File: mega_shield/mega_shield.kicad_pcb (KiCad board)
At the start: 2 copper layers, 296 parts, among them J11 T4040014031-000, J13 T4040014031-000, J14 1757242, J15 1757242, J17 T4040014031-000, J19 T4040014031-000, J20 T4140012121-000, J3 1757271, J9 T4040014031-000, Q1 2SK3018, Q10 2SK3018, Q11 2SK3018, Q12 2SK3018, Q13 2SK3018, Q14 2SK3018, Q15 2SK3018, Q16 2SK3018, Q17 2SK3018, Q18 2SK3018, Q19 2SK3018, Q2 2SK3018, Q20 2SK3018, Q21 2SK3018, Q22 2SK3018, Q23 2SK3018, Q24 2SK3018, Q25 2SK3018, Q26 2SK3018, Q27 2SK3018, Q28 2SK3018, Q29 2SK3018, Q3 2SK3018, Q30 2SK3018, Q31 2SK3018, Q32 2SK3018, Q33 2SK3018, Q34 2SK3018, Q35 2SK3018, Q36 2SK3018, Q37 2SK3018, Q38 2SK3018, Q39 2SK3018, Q4 2SK3018, Q40 2SK3018, Q41 2SK3018, Q42 2SK3018, Q5 2SK3018, Q6 2SK3018, Q7 2SK3018, Q8 2SK3018, Q9 2SK3018, U1 CS817x22HS, U10 CS817x22HS, U11 CS817x22HS, U12 CS817x22HS, U13 CS817x22HS, U14 CS817x22HS, U15 CS817x22HS, U16 CS817x22HS, U17 CS817x22HS, U18 CS817x22HS, U19 NUP2202, U2 CS817x22HS, U20 NUP2202, U21 NUP2202, U22 NUP2202, U23 NUP2202, U24 CS817x22HS, U25 CS817x22HS, U26 CS817x22HS, U27 CS817x22HS, U28 CS817x22HS, U3 CS817x22HS, U4 CS817x22HS, U5 CS817x22HS, U6 CS817x22HS, U7 MCP6241RT-I-OT, U8 NUP2202, U9 CS817x22HS

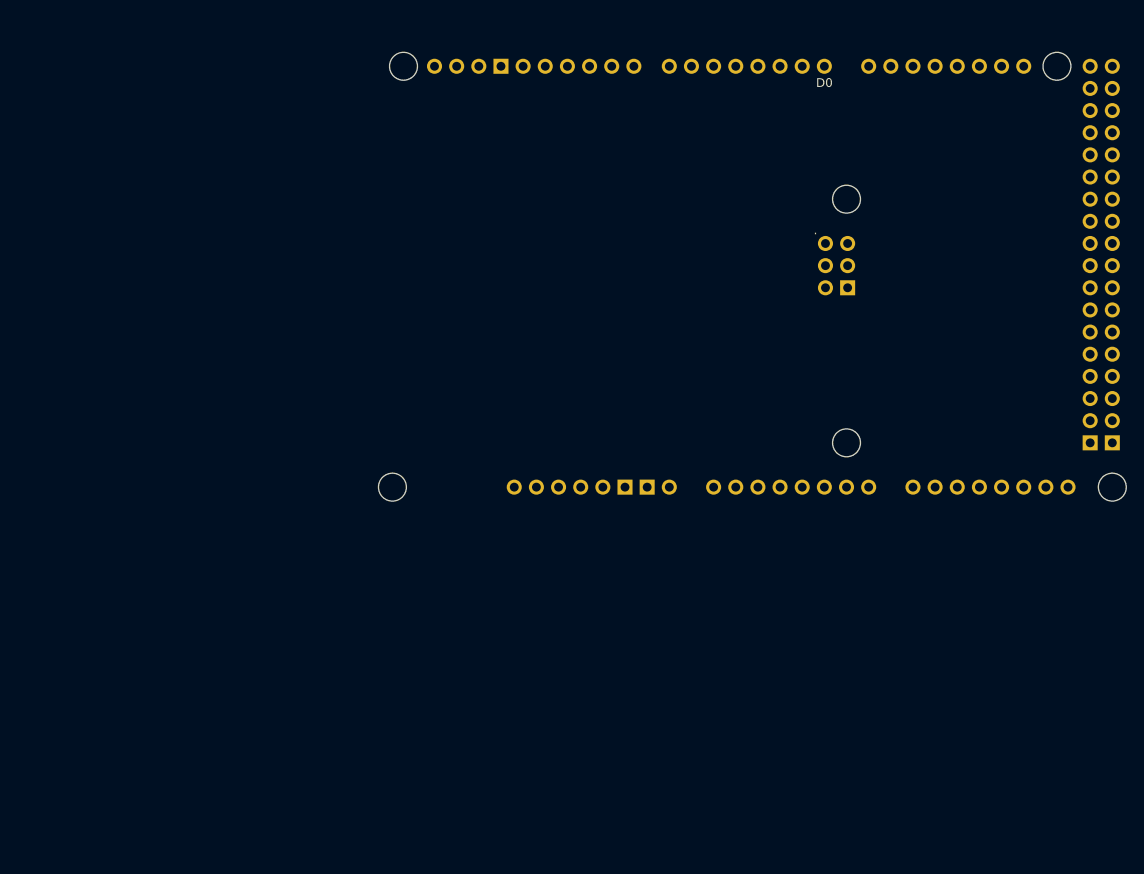
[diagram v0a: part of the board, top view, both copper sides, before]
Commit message: moved mega shield to x:75, y:150
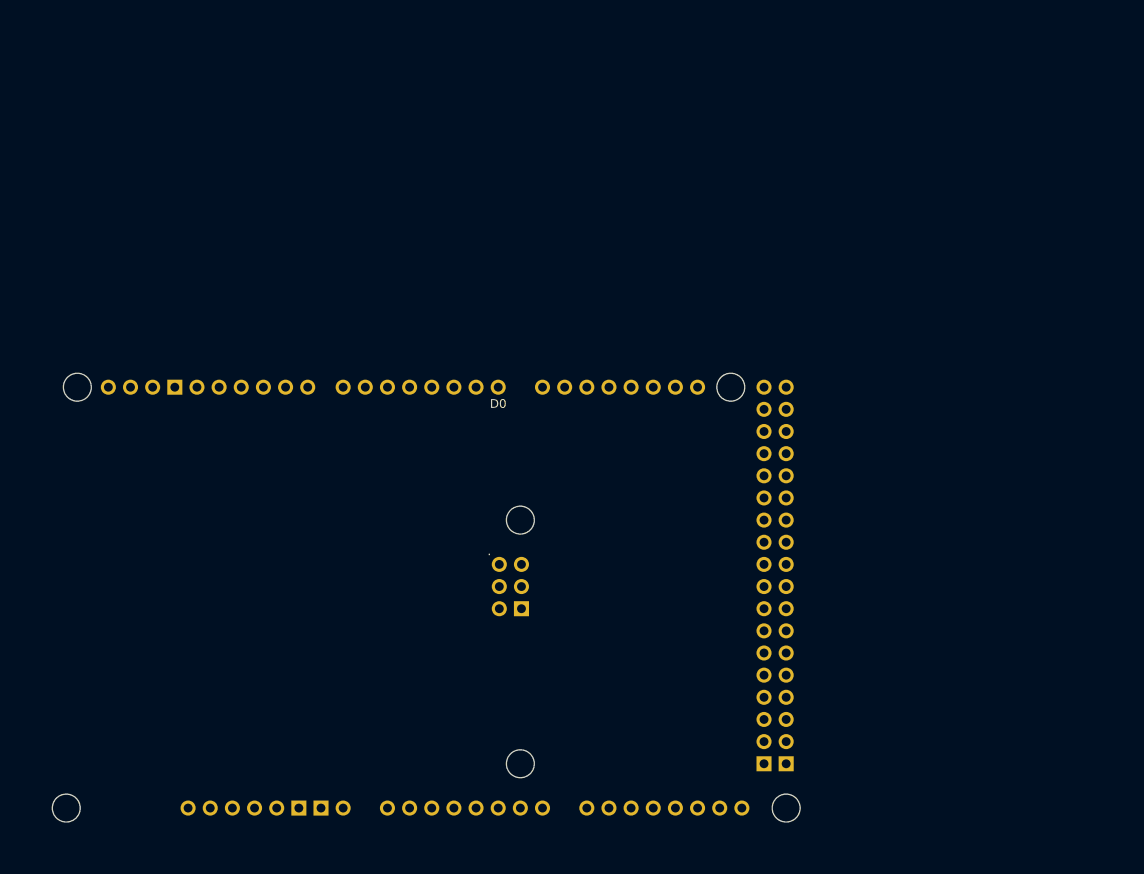
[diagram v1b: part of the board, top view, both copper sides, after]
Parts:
- moved A1 52.5 mm to (75.0, 150.0)
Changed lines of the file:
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@@
 		(legacy_teardrops no)
 	)
-	(paper "A4")
+	(paper "A3")
 	(layers
 		(0 "F.Cu" signal)
@@
 	(footprint "PCM_arduino-library:Arduino_Mega2560_R3_Shield"
 		(layer "F.Cu")
-		(at 112.4 113.2)
+		(at 75 150)
 		(descr "https://docs.arduino.cc/hardware/mega-2560")
 		(property "Reference" "A1"
